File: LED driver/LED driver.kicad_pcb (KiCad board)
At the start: 2 copper layers, 57.5 x 41 mm, 45 parts, among them J1 Conn_VCC_Alt, J2 Conn_VCC, J3 Conn_LED, J4 Conn_Boot_Mode, J5 Conn_UART, J6 Conn_Aux, Q1 ZXMN3A01F, Q2 ZXMN3A01F, Q3 ZXMN3A01F, Q4 ZXMN3A01F, Q5 ZXMN3A01F, SW1 SW_Push, U1 ESP32-C3-WROOM-02, U2 MP2359

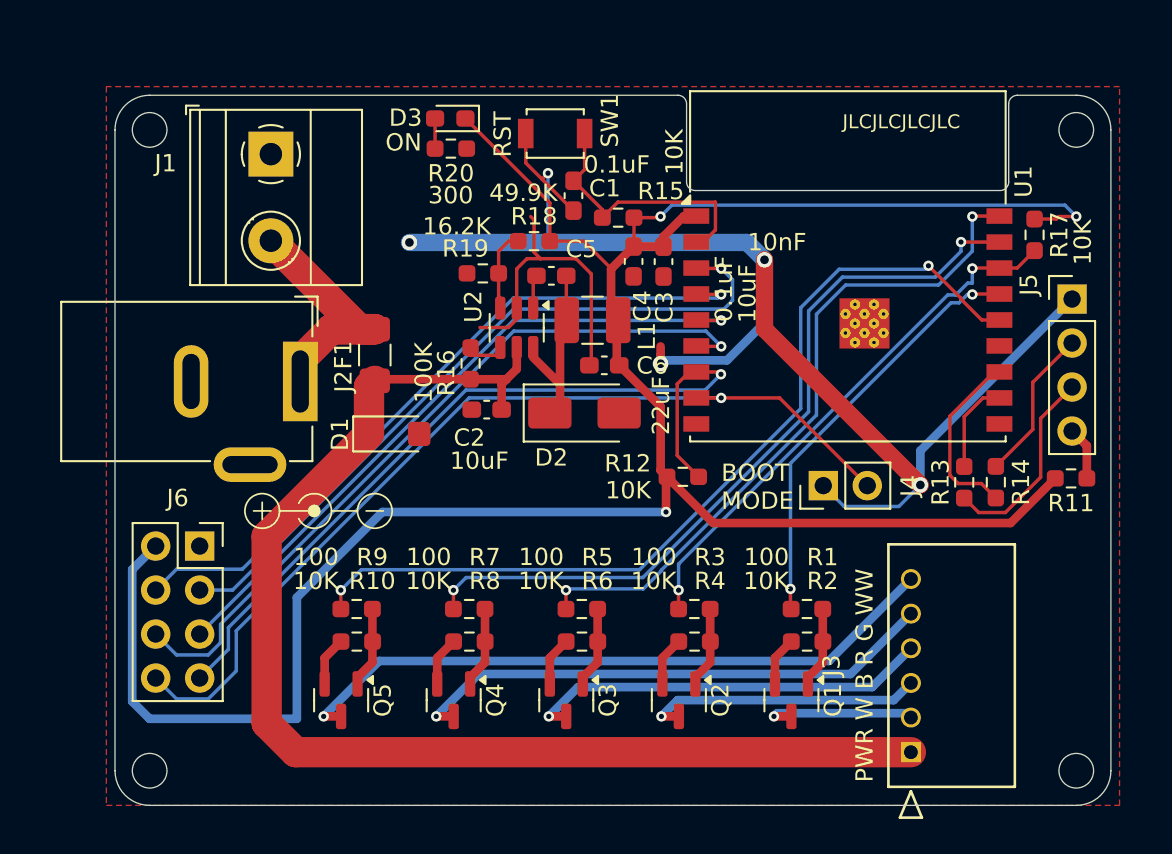
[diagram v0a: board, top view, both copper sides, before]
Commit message: 2024-04-13
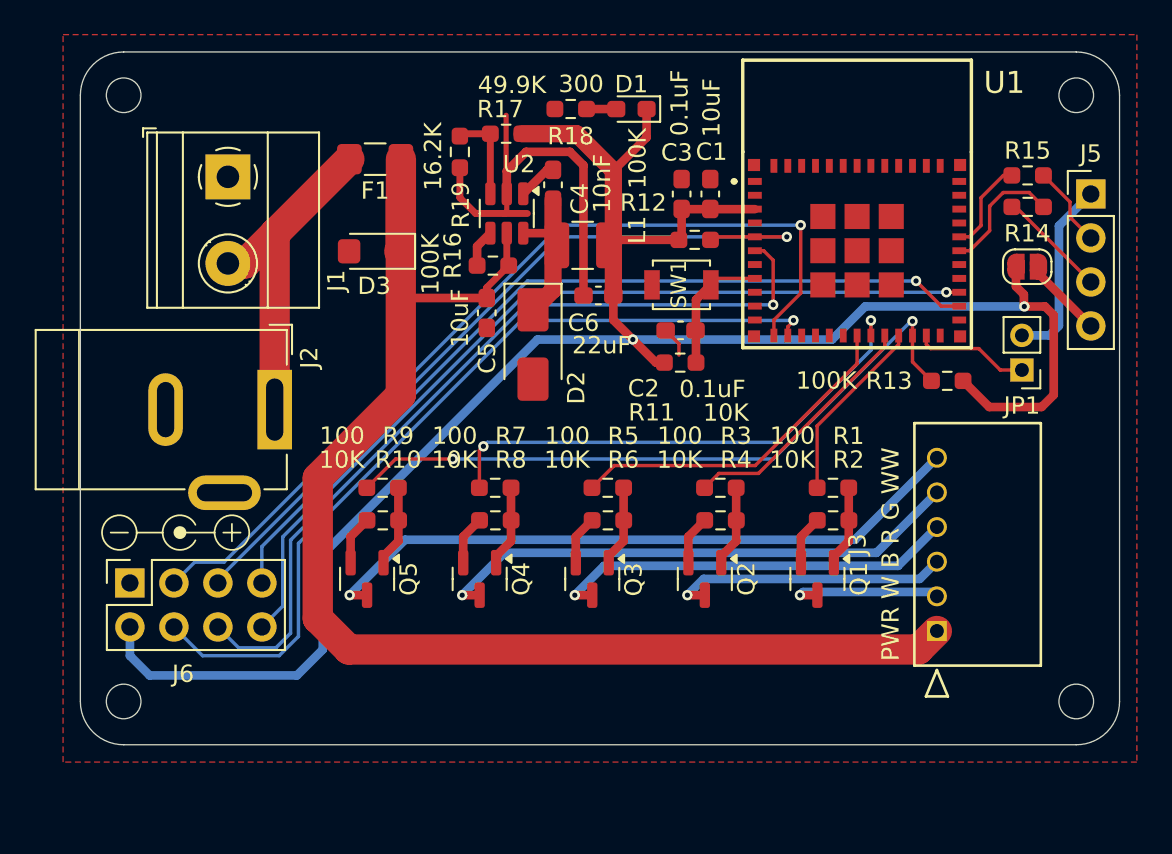
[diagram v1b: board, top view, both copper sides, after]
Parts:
- removed J4: Conn_Boot_Mode, Connector_PinHeader_2.54mm:PinHeader_1x02_P2.54mm_Vertical
- removed R20: 300, Custom:R_0603_HandSolder_ValuePrinted
- added JP1: Boot_Mode, Connector_PinHeader_2.00mm:PinHeader_1x02_P2.00mm_Vertical, F.Cu at (151.7, 73.4)
- added JP2: SolderJumper_2_Open, Jumper:SolderJumper-2_P1.3mm_Open_RoundedPad1.0x1.5mm, F.Cu at (152.0, 67.5)
- C1: value 0.1uF -> 10uF
- C2, C3: value 10uF -> 0.1uF
- C4: value 0.1uF -> 10nF
- C5: value 10nF -> 10uF
- D1: value SMF24A -> PWR_LED; footprint Diode_SMD:D_SMF -> Diode_SMD:D_0603_1608Metric_Pad1.05x0.95mm_HandSolder
- D3: value PWR_LED -> SMF24A; footprint Diode_SMD:D_0603_1608Metric_Pad1.05x0.95mm_HandSolder -> Diode_SMD:D_SMF
- J2: footprint Connector_BarrelJack:BarrelJack_GCT_DCJ200-10-A_Horizontal -> Custom:BarrelJack_GCT_DCJ200-10-A_Horizontal
- R11: value 0 -> 10K; footprint Resistor_SMD:R_0603_1608Metric_Pad0.98x0.95mm_HandSolder -> Custom:R_0603_HandSolder_ValuePrinted
- R12: value 10K -> 100K
- R13: value 0 -> 100K; footprint Resistor_SMD:R_0603_1608Metric_Pad0.98x0.95mm_HandSolder -> Custom:R_0603_HandSolder_ValuePrinted
- R15: value 10K -> 0; footprint Custom:R_0603_HandSolder_ValuePrinted -> Resistor_SMD:R_0603_1608Metric_Pad0.98x0.95mm_HandSolder
- R17: value 10K -> 49.9K
- R18: value 49.9K -> 300
- U1: value ESP32-C3-WROOM-02 -> ESP32-C3-MINI-1-N4; footprint RF_Module:ESP32-C3-WROOM-02 -> ESP32-C3-MINI-1-N4:ESP32C3MINI1N4
- moved R17 31.1 mm to (121.9, 59.8), turned to 0 degrees
- moved R15 23.8 mm to (152.0, 62.2), turned to 0 degrees
- moved R11 23.5 mm to (131.9, 73.0), turned to 0 degrees
- moved D1 23.2 mm to (129.1, 58.4), turned to 180 degrees
- moved R14 16.0 mm to (152.0, 64.0), turned to 180 degrees
- moved R12 13.7 mm to (132.8, 65.9)
- moved C2 12.1 mm to (132.0, 71.2), turned to 0 degrees
- moved SW1 11.4 mm to (132.0, 68.5)
- moved F1 11.3 mm to (114.3, 61.3), turned to 180 degrees
- moved D3 8.84 mm to (114.3, 66.6)
- moved R18 7.92 mm to (125.6, 58.4)
- moved C1 7.90 mm to (133.7, 63.3), turned to -90 degrees
- moved J3 7.16 mm to (146.8, 88.5)
- moved Q1 7.16 mm to (139.9, 85.5)
- moved Q2 7.16 mm to (133.4, 85.5)
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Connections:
- net /IO7 renamed /IO3
- C1 pad 2: Net-(U1-EN) -> +3.3V
- C2 pad 1: VCC -> GND
- C2 pad 2: GND -> Net-(U1-EN)
- C4 pad 1: GND -> Net-(U2-BST)
- C4 pad 2: +3.3V -> Net-(D2-K)
- C5 pad 1: Net-(U2-BST) -> VCC
- C5 pad 2: Net-(D2-K) -> GND
- D1 pad 1: VCC -> +3.3V
- D1 pad 2: GND -> Net-(D1-A)
- D3 pad 1: +3.3V -> VCC
- D3 pad 2: Net-(D3-A) -> GND
- J5 pad 2: /TX -> Net-(J5-Pin_2)
- J5 pad 3: /RX -> Net-(J5-Pin_3)
- J6 pad 3: /IO4 -> /IO0
- J6 pad 4: /IO5 -> /IO1
- J6 pad 5: /IO6 -> /IO2
- J6 pad 7: /IO8 -> /IO18
- J6 pad 8: /IO9 -> /IO19
- R11 pad 1: Net-(J5-Pin_4) -> +3.3V
- R11 pad 2: +3.3V -> Net-(U1-EN)
- R12 pad 2: /IO8 -> /IO2
- R13 pad 1: Net-(U1-RXD) -> +3.3V
- R13 pad 2: /RX -> /PWM_WW
- R14 pad 1: Net-(U1-TXD) -> /RX
- R14 pad 2: /TX -> Net-(J5-Pin_3)
- R15 pad 1: +3.3V -> /TX
- R15 pad 2: Net-(U1-EN) -> Net-(J5-Pin_2)
- R17 pad 1: +3.3V -> Net-(U2-FB)
- R17 pad 2: /PWM_B -> +3.3V
- R18 pad 1: Net-(U2-FB) -> GND
- R18 pad 2: +3.3V -> Net-(D1-A)
- U1 pad 1: +3.3V -> GND
- U1 pad 11: Net-(U1-RXD) -> GND
- U1 pad 12: Net-(U1-TXD) -> /IO0
- U1 pad 13: unconnected-(U1-IO18-Pad13) -> /IO1
- U1 pad 14: /PWM_WW -> GND
- U1 pad 15: /PWM_W -> unconnected-(U1-NC_5-Pad15)
- U1 pad 16: /PWM_B -> unconnected-(U1-IO10-Pad16)
- U1 pad 17: /PWM_G -> unconnected-(U1-NC_6-Pad17)
- U1 pad 19: GND -> /PWM_G
- U1 pad 2: Net-(U1-EN) -> GND
- U1 pad 3: /IO4 -> +3.3V
- U1 pad 4: /IO5 -> unconnected-(U1-NC_1-Pad4)
- U1 pad 5: /IO6 -> /IO2
- U1 pad 7: /IO8 -> unconnected-(U1-NC_2-Pad7)
- U1 pad 8: /IO9 -> Net-(U1-EN)
- U1 pad 9: GND -> unconnected-(U1-NC_3-Pad9)
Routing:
- net GND: track 112.1 -> 52.4 mm, vias 5 -> 0
- net /IO0: track 0.00 -> 51.8 mm, vias 0 -> 1
- net /IO19: track 0.00 -> 50.6 mm, vias 0 -> 1
- net /IO18: track 0.00 -> 49.3 mm, vias 0 -> 1
- net /IO1: track 0.00 -> 48.6 mm, vias 0 -> 1
- net /IO9: track 53.7 -> 6.64 mm, vias 1 -> 0
- net /IO8: track 46.8 -> 0.00 mm, vias 1 -> 0
- net /IO2: track 0.00 -> 45.7 mm, vias 0 -> 1
- net /IO4: track 41.3 -> 0.00 mm, vias 1 -> 0
- net /IO5: track 41.2 -> 0.00 mm, vias 1 -> 0
- net /IO6: track 39.1 -> 0.00 mm, vias 1 -> 0
- net +3.3V: track 143.0 -> 114.4 mm, vias 3 -> 2
- net /PWM_R: track 39.7 -> 19.9 mm, vias 2 -> 0
- net /PWM_B: track 31.1 -> 14.4 mm, vias 2 -> 0
- net /PWM_G: track 44.7 -> 29.8 mm
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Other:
- board size 57.5 x 41 mm -> 60 x 40 mm
- board text removed: "BOOT MODE"
- board text removed: "JLCJLCJLCJLC"
- board text removed: "ON"
- board text removed: "RST"
